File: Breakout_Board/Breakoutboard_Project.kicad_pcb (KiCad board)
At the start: 2 copper layers, 60 x 60 mm, 36 parts, among them J1 Conn_01x17, J2 Conn_01x17, J3 Conn_02x06_Top_Bottom, J4 Conn_01x05, U1 ADXL380-2BCCZ-RL7, U2 STM32F411, U3 ICM-40609-D, U4 MMC5983MA, U5 BMP585

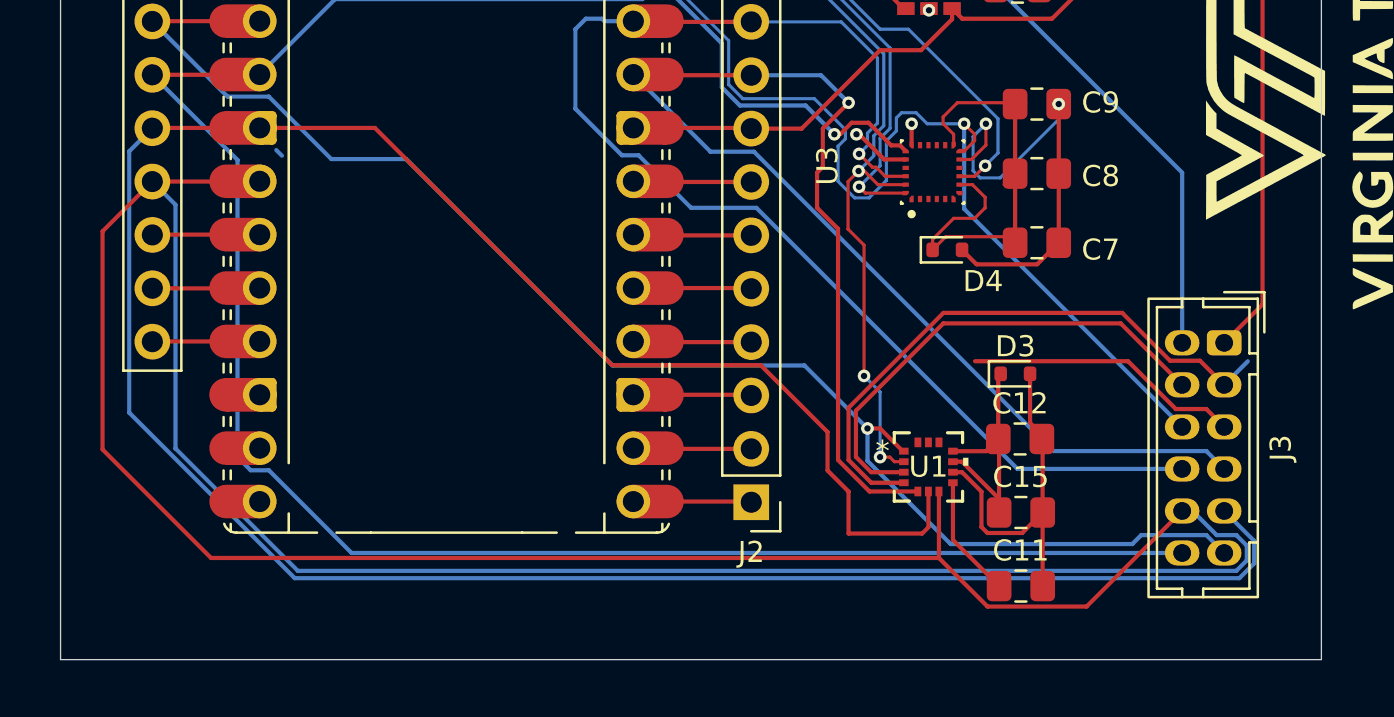
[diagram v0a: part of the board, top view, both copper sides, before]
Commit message: clicked b
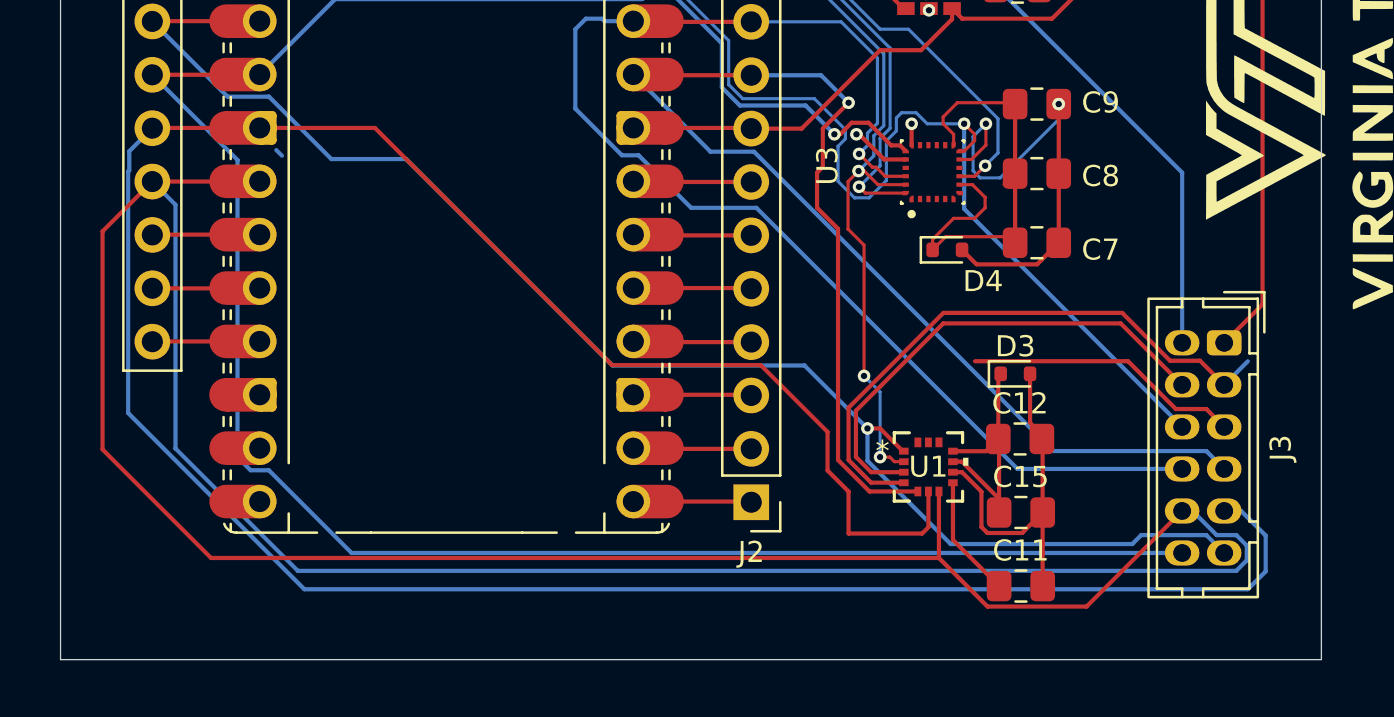
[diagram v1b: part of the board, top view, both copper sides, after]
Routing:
- net /ADXL_INT0: track 123.2 -> 125.2 mm
